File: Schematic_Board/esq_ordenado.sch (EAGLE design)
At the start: 52 parts, among them IC1 LM1117IMPX-3.3, Q1 SMD-TRANSISTORS-NPN-25V-500MW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, Q2 SMD-TRANSISTORS-NPN-25V-500MW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, U1 ESP-32S, U2 CP2102-GM, U3 TPD2S017DBVR, U4 Value, U5 TMP275AIDR

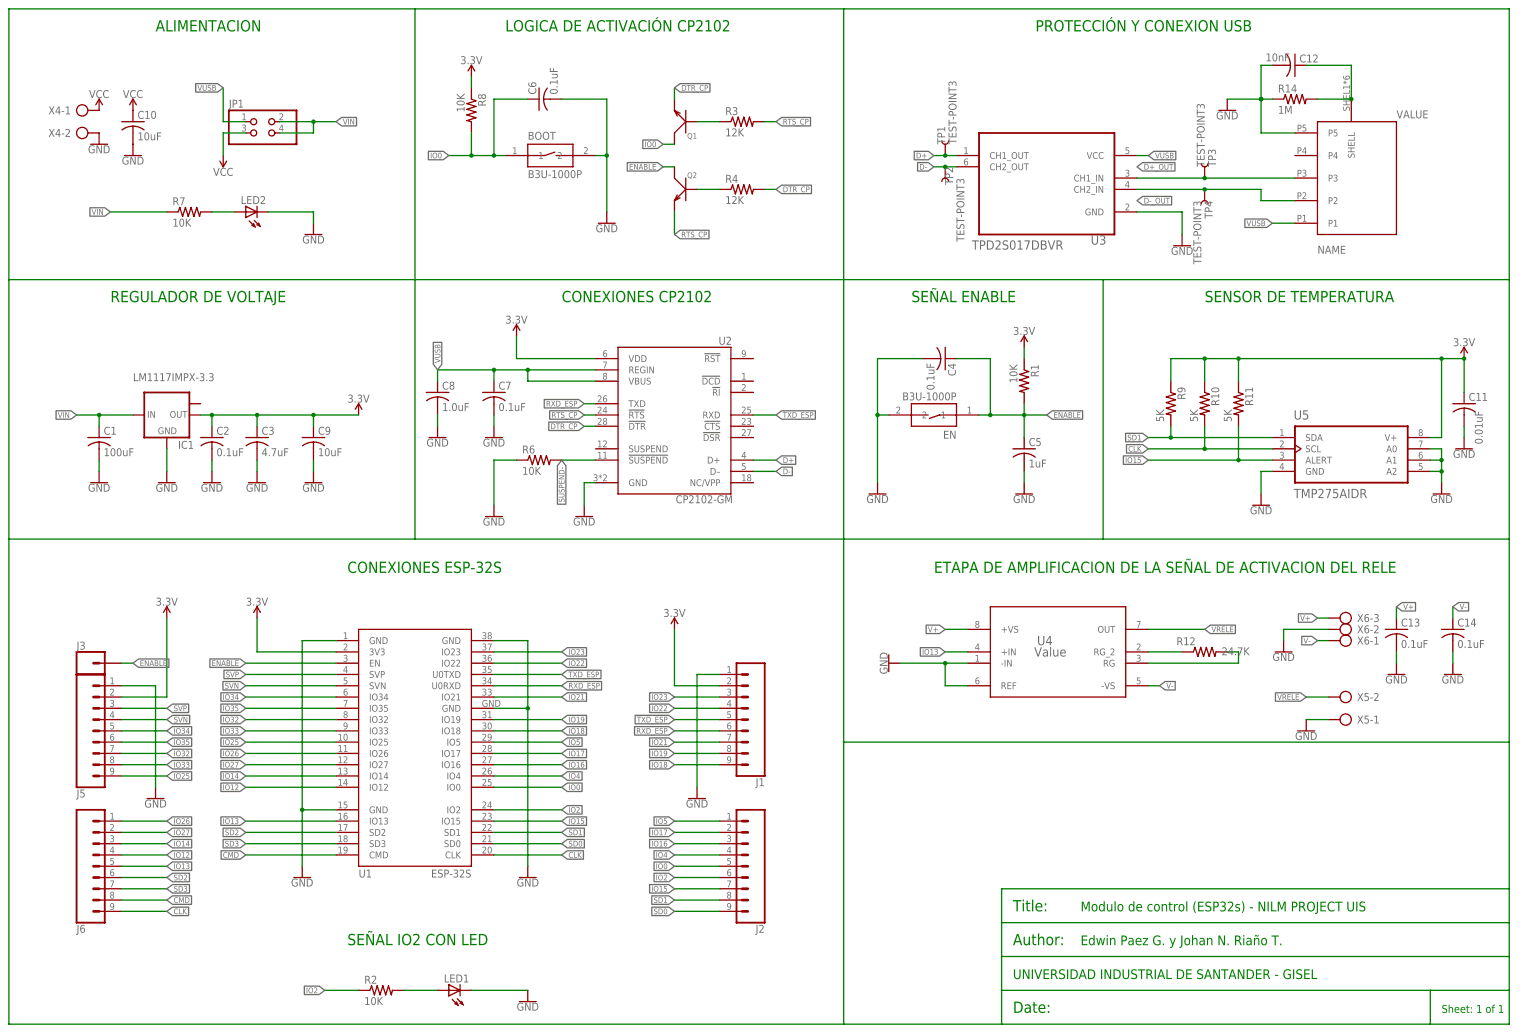
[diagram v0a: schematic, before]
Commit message: Correc Borneras - revision nicolas
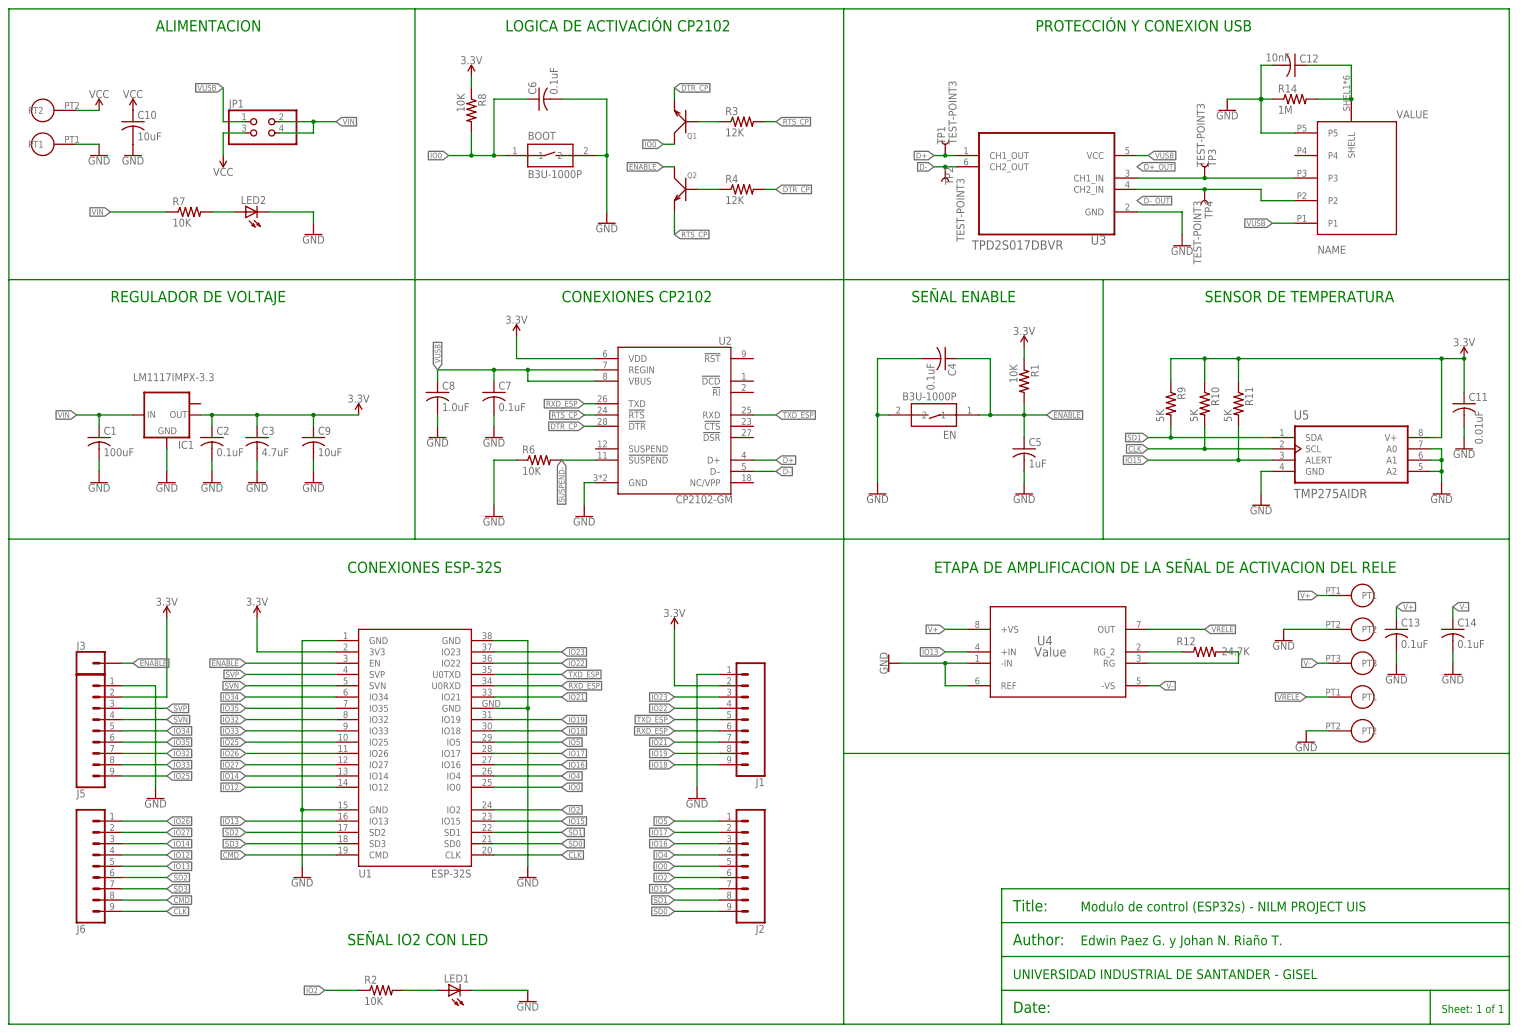
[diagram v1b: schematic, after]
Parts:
- removed X4, X5: (no value), con-ptr500:AK500/2
- removed X6: (no value), con-ptr500:AK500/3
- added U$2, U$3: PT2,5/2-5,0, con_phoenix:PT2,5/2-5,0
- added U$4: PT2,5/3-5,0, con_phoenix:PT2,5/3-5,0
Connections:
- net GND: now also U$2.PT1, U$3.PT2, U$4.PT2; no longer X4-2.KL, X5-1.KL, X6-2.KL
- net V+: now also U$4.PT1; no longer X6-3.KL
- net V-: now also U$4.PT3; no longer X6-1.KL
- net VCC: now also U$2.PT2; no longer X4-1.KL
- net VRELE: now also U$3.PT1; no longer X5-2.KL
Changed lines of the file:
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@@
 <part name="GND15" library="SparkFun-PowerSymbols" library_urn="urn:adsk.eagle:library:530" deviceset="GND" device=""/>
 <part name="GND30" library="SparkFun-PowerSymbols" library_urn="urn:adsk.eagle:library:530" deviceset="GND" device=""/>
-<part name="X4" library="con-ptr500" library_urn="urn:adsk.eagle:library:181" deviceset="AK500/2" device="" package3d_urn="urn:adsk.eagle:package:9880/1"/>
-<part name="X5" library="con-ptr500" library_urn="urn:adsk.eagle:library:181" deviceset="AK500/2" device="" package3d_urn="urn:adsk.eagle:package:9880/1"/>
-<part name="X6" library="con-ptr500" library_urn="urn:adsk.eagle:library:181" deviceset="AK500/3" device="" package3d_urn="urn:adsk.eagle:package:9883/1"/>
+<part name="U$2" library="con_phoenix" deviceset="PT2,5/2-5,0" device=""/>
+<part name="U$3" library="con_phoenix" deviceset="PT2,5/2-5,0" device=""/>
+<part name="U$4" library="con_phoenix" deviceset="PT2,5/3-5,0" device=""/>
 </parts>
 <sheets>
@@
 <attribute name="VALUE" x="20.32" y="208.534" size="1.778" layer="96" align="bottom-center"/>
 </instance>
-<instance part="GND8" gate="1" x="20.32" y="198.12" smashed="yes">
-<attribute name="VALUE" x="20.32" y="197.866" size="1.778" layer="96" align="top-center"/>
+<instance part="GND8" gate="1" x="20.32" y="195.58" smashed="yes">
+<attribute name="VALUE" x="20.32" y="195.326" size="1.778" layer="96" align="top-center"/>
 </instance>
 <instance part="C2" gate="G$1" x="45.72" y="132.08" smashed="yes">
@@
 <attribute name="VALUE" x="197.866" y="81.28" size="1.778" layer="96" rot="R270" align="top-center"/>
 </instance>
-<instance part="GND29" gate="1" x="287.02" y="83.82" smashed="yes">
-<attribute name="VALUE" x="287.02" y="83.566" size="1.778" layer="96" align="top-center"/>
+<instance part="GND29" gate="1" x="287.02" y="86.36" smashed="yes">
+<attribute name="VALUE" x="287.02" y="86.106" size="1.778" layer="96" align="top-center"/>
 </instance>
 <instance part="U$1" gate="G$1" x="302.26" y="187.96" smashed="yes" rot="MR180"/>
@@
 <attribute name="VALUE" x="273.05" y="83.058" size="1.778" layer="96"/>
 </instance>
-<instance part="GND14" gate="1" x="292.1" y="66.04" smashed="yes">
-<attribute name="VALUE" x="292.1" y="65.786" size="1.778" layer="96" align="top-center"/>
+<instance part="GND14" gate="1" x="292.1" y="63.5" smashed="yes">
+<attribute name="VALUE" x="292.1" y="63.246" size="1.778" layer="96" align="top-center"/>
 </instance>
 <instance part="BOOT" gate="G$1" x="121.92" y="195.58" smashed="yes">
@@
 <attribute name="VALUE" x="325.12" y="78.486" size="1.778" layer="96" align="top-center"/>
 </instance>
-<instance part="X4" gate="-1" x="15.24" y="205.74" smashed="yes">
-<attribute name="NAME" x="13.97" y="206.629" size="1.778" layer="95" rot="R180"/>
-</instance>
-<instance part="X4" gate="-2" x="15.24" y="200.66" smashed="yes">
-<attribute name="NAME" x="13.97" y="201.549" size="1.778" layer="95" rot="R180"/>
-<attribute name="VALUE" x="11.43" y="196.977" size="1.778" layer="96"/>
-</instance>
-<instance part="X5" gate="-1" x="302.26" y="68.58" smashed="yes" rot="R180">
-<attribute name="NAME" x="303.53" y="67.691" size="1.778" layer="95"/>
-</instance>
-<instance part="X5" gate="-2" x="302.26" y="73.66" smashed="yes" rot="R180">
-<attribute name="NAME" x="303.53" y="72.771" size="1.778" layer="95"/>
-<attribute name="VALUE" x="306.07" y="77.343" size="1.778" layer="96" rot="R180"/>
-</instance>
-<instance part="X6" gate="-1" x="302.26" y="86.36" smashed="yes" rot="R180">
-<attribute name="NAME" x="303.53" y="85.471" size="1.778" layer="95"/>
-</instance>
-<instance part="X6" gate="-2" x="302.26" y="88.9" smashed="yes" rot="R180">
-<attribute name="NAME" x="303.53" y="88.011" size="1.778" layer="95"/>
-</instance>
-<instance part="X6" gate="-3" x="302.26" y="91.44" smashed="yes" rot="R180">
-<attribute name="NAME" x="303.53" y="90.551" size="1.778" layer="95"/>
-<attribute name="VALUE" x="306.07" y="95.123" size="1.778" layer="96" rot="R180"/>
-</instance>
+<instance part="U$2" gate="G$1" x="10.16" y="198.12" smashed="yes" rot="R180"/>
+<instance part="U$3" gate="G$1" x="302.26" y="73.66" smashed="yes"/>
+<instance part="U$4" gate="G$1" x="302.26" y="88.9" smashed="yes"/>
 </instances>
 <busses>
@@
 </segment>
 <segment>
+<pinref part="U$2" gate="G$1" pin="PT2"/>
 <pinref part="SUPPLY6" gate="G$1" pin="VCC"/>
-<pinref part="X4" gate="-1" pin="KL"/>
+<wire x1="15.24" y1="205.74" x2="20.32" y2="205.74" width="0.1524" layer="91"/>
 </segment>
 </net>
@@
 <segment>
 <wire x1="297.18" y1="88.9" x2="287.02" y2="88.9" width="0.1524" layer="91"/>
-<wire x1="287.02" y1="88.9" x2="287.02" y2="86.36" width="0.1524" layer="91"/>
 <pinref part="GND29" gate="1" pin="GND"/>
-<pinref part="X6" gate="-2" pin="KL"/>
-</segment>
-<segment>
-<wire x1="297.18" y1="68.58" x2="292.1" y2="68.58" width="0.1524" layer="91"/>
+<pinref part="U$4" gate="G$1" pin="PT2"/>
+</segment>
+<segment>
+<wire x1="297.18" y1="66.04" x2="292.1" y2="66.04" width="0.1524" layer="91"/>
 <pinref part="GND14" gate="1" pin="GND"/>
-<pinref part="X5" gate="-1" pin="KL"/>
+<pinref part="U$3" gate="G$1" pin="PT2"/>
 </segment>
 <segment>
@@
 </segment>
 <segment>
+<pinref part="U$2" gate="G$1" pin="PT1"/>
 <pinref part="GND8" gate="1" pin="GND"/>
-<pinref part="X4" gate="-2" pin="KL"/>
+<wire x1="15.24" y1="198.12" x2="20.32" y2="198.12" width="0.1524" layer="91"/>
 </segment>
 </net>
@@
 <wire x1="187.96" y1="167.64" x2="187.96" y2="109.22" width="0.1524" layer="91"/>
 <wire x1="0" y1="167.64" x2="187.96" y2="167.64" width="0.1524" layer="91"/>
-<wire x1="187.96" y1="109.22" x2="187.96" y2="63.5" width="0.1524" layer="91"/>
-<wire x1="187.96" y1="63.5" x2="187.96" y2="0" width="0.1524" layer="91"/>
+<wire x1="187.96" y1="109.22" x2="187.96" y2="60.96" width="0.1524" layer="91"/>
+<wire x1="187.96" y1="60.96" x2="187.96" y2="0" width="0.1524" layer="91"/>
 <wire x1="187.96" y1="167.64" x2="246.38" y2="167.64" width="0.1524" layer="91"/>
 <wire x1="246.38" y1="167.64" x2="337.82" y2="167.64" width="0.1524" layer="91"/>
@@
 <wire x1="337.82" y1="15.24" x2="337.82" y2="22.86" width="0.1524" layer="91"/>
 <wire x1="337.82" y1="22.86" x2="337.82" y2="30.48" width="0.1524" layer="91"/>
-<wire x1="337.82" y1="30.48" x2="337.82" y2="63.5" width="0.1524" layer="91"/>
-<wire x1="337.82" y1="63.5" x2="337.82" y2="109.22" width="0.1524" layer="91"/>
+<wire x1="337.82" y1="30.48" x2="337.82" y2="60.96" width="0.1524" layer="91"/>
+<wire x1="337.82" y1="60.96" x2="337.82" y2="109.22" width="0.1524" layer="91"/>
 <wire x1="337.82" y1="109.22" x2="337.82" y2="167.64" width="0.1524" layer="91"/>
 <wire x1="187.96" y1="109.22" x2="246.38" y2="109.22" width="0.1524" layer="91"/>
 <wire x1="246.38" y1="109.22" x2="246.38" y2="167.64" width="0.1524" layer="91"/>
 <wire x1="246.38" y1="109.22" x2="337.82" y2="109.22" width="0.1524" layer="91"/>
-<wire x1="187.96" y1="63.5" x2="337.82" y2="63.5" width="0.1524" layer="91"/>
+<wire x1="187.96" y1="60.96" x2="337.82" y2="60.96" width="0.1524" layer="91"/>
 <wire x1="223.52" y1="30.48" x2="337.82" y2="30.48" width="0.1524" layer="91"/>
 <wire x1="223.52" y1="30.48" x2="223.52" y2="22.86" width="0.1524" layer="91"/>
@@
 <wire x1="297.18" y1="73.66" x2="292.1" y2="73.66" width="0.1524" layer="91"/>
 <label x="292.1" y="73.66" size="1.27" layer="95" rot="R180" xref="yes"/>
-<pinref part="X5" gate="-2" pin="KL"/>
+<pinref part="U$3" gate="G$1" pin="PT1"/>
 </segment>
 </net>
@@
 </segment>
 <segment>
-<wire x1="297.18" y1="86.36" x2="294.64" y2="86.36" width="0.1524" layer="91"/>
-<label x="294.64" y="86.36" size="1.27" layer="95" rot="R180" xref="yes"/>
-<pinref part="X6" gate="-1" pin="KL"/>
+<wire x1="297.18" y1="81.28" x2="294.64" y2="81.28" width="0.1524" layer="91"/>
+<label x="294.64" y="81.28" size="1.27" layer="95" rot="R180" xref="yes"/>
+<pinref part="U$4" gate="G$1" pin="PT3"/>
 </segment>
 <segment>
@@
 </segment>
 <segment>
-<wire x1="297.18" y1="91.44" x2="294.64" y2="91.44" width="0.1524" layer="91"/>
-<label x="294.64" y="91.44" size="1.27" layer="95" rot="R180" xref="yes"/>
-<pinref part="X6" gate="-3" pin="KL"/>
-</segment>
-<segment>
+<wire x1="297.18" y1="96.52" x2="294.64" y2="96.52" width="0.1524" layer="91"/>
+<label x="294.64" y="96.52" size="1.27" layer="95" rot="R180" xref="yes"/>
+<pinref part="U$4" gate="G$1" pin="PT1"/>
+</segment>
+<segment>
